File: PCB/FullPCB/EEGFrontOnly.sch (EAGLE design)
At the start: 208 parts, among them IC1 ADS1299-X, IC2 ADUM4160BRWZ, J11 MICRO-SD_CARD_SOCKET, J12 455-1750-1-ND, J13 455-1750-1-ND, J14 455-1750-1-ND, J15 455-1750-1-ND, J2 USB_B_PTH, J8 JTAG, U1 LP2985-33DBVT, U10 HT7318, U11 TMS320F28335PGFA, U12 HT7333, U13 2.93V, U14 MAX811-812, U2 B0505S-1WB0505S-1W, U3 TPS60403DBVT, U4 TPS73225DBVR, U5 TPS73225DBVR, U6 TPD4E1B06DCKR, U7 TPD4E1B06DCKR, U8 TPD4E1B06DCKR, U9 HT7333, Y1 30MHz, Y2 12MHz

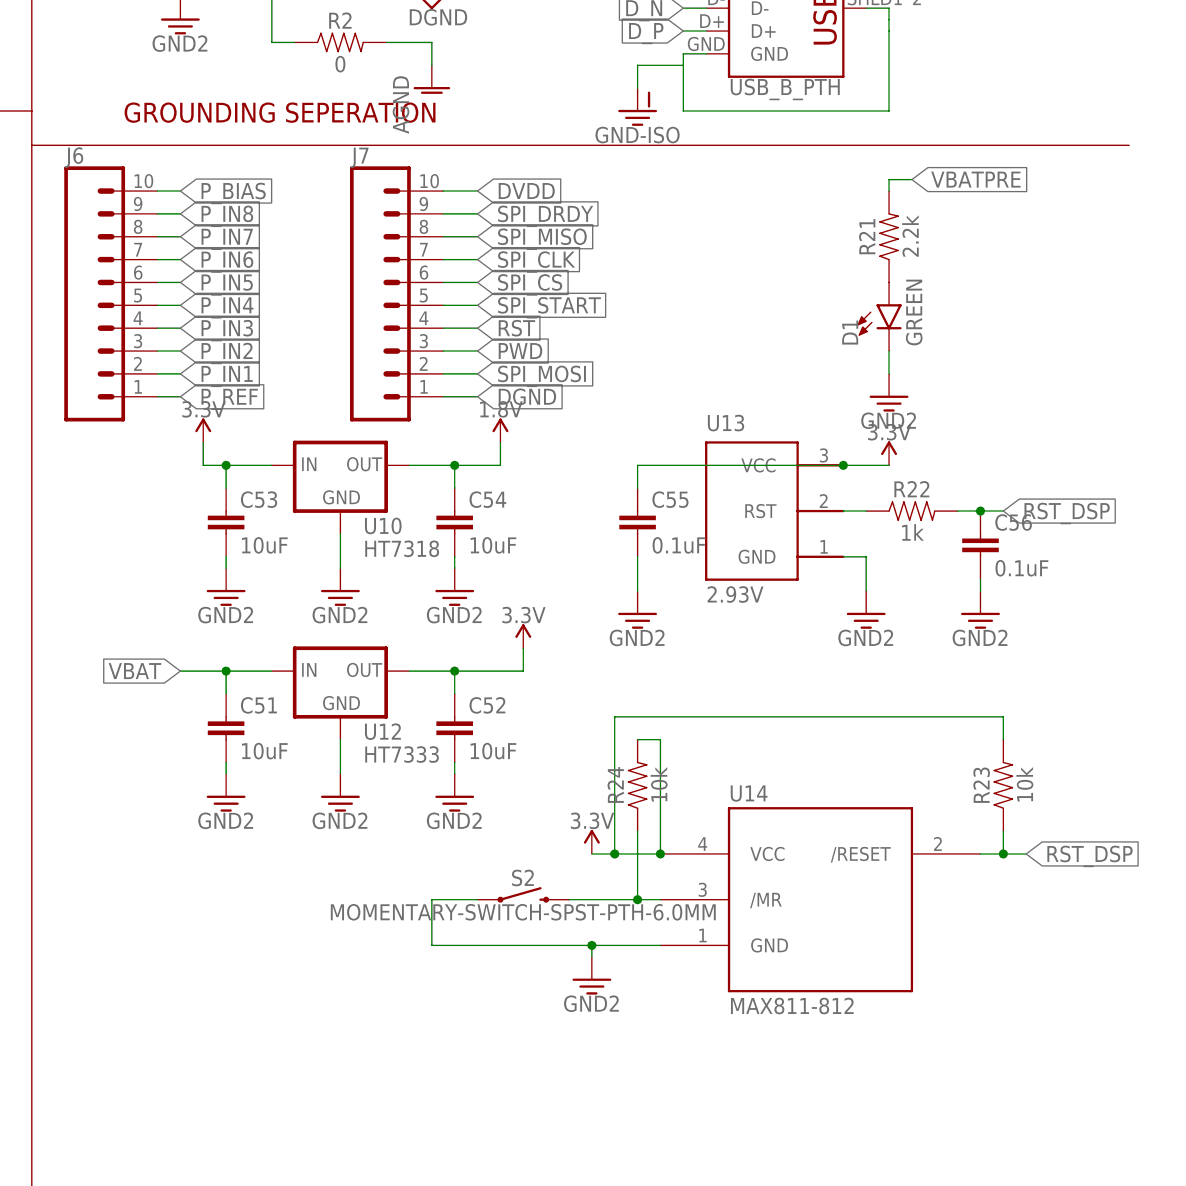
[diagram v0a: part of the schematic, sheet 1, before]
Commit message: full pcb nearly complete
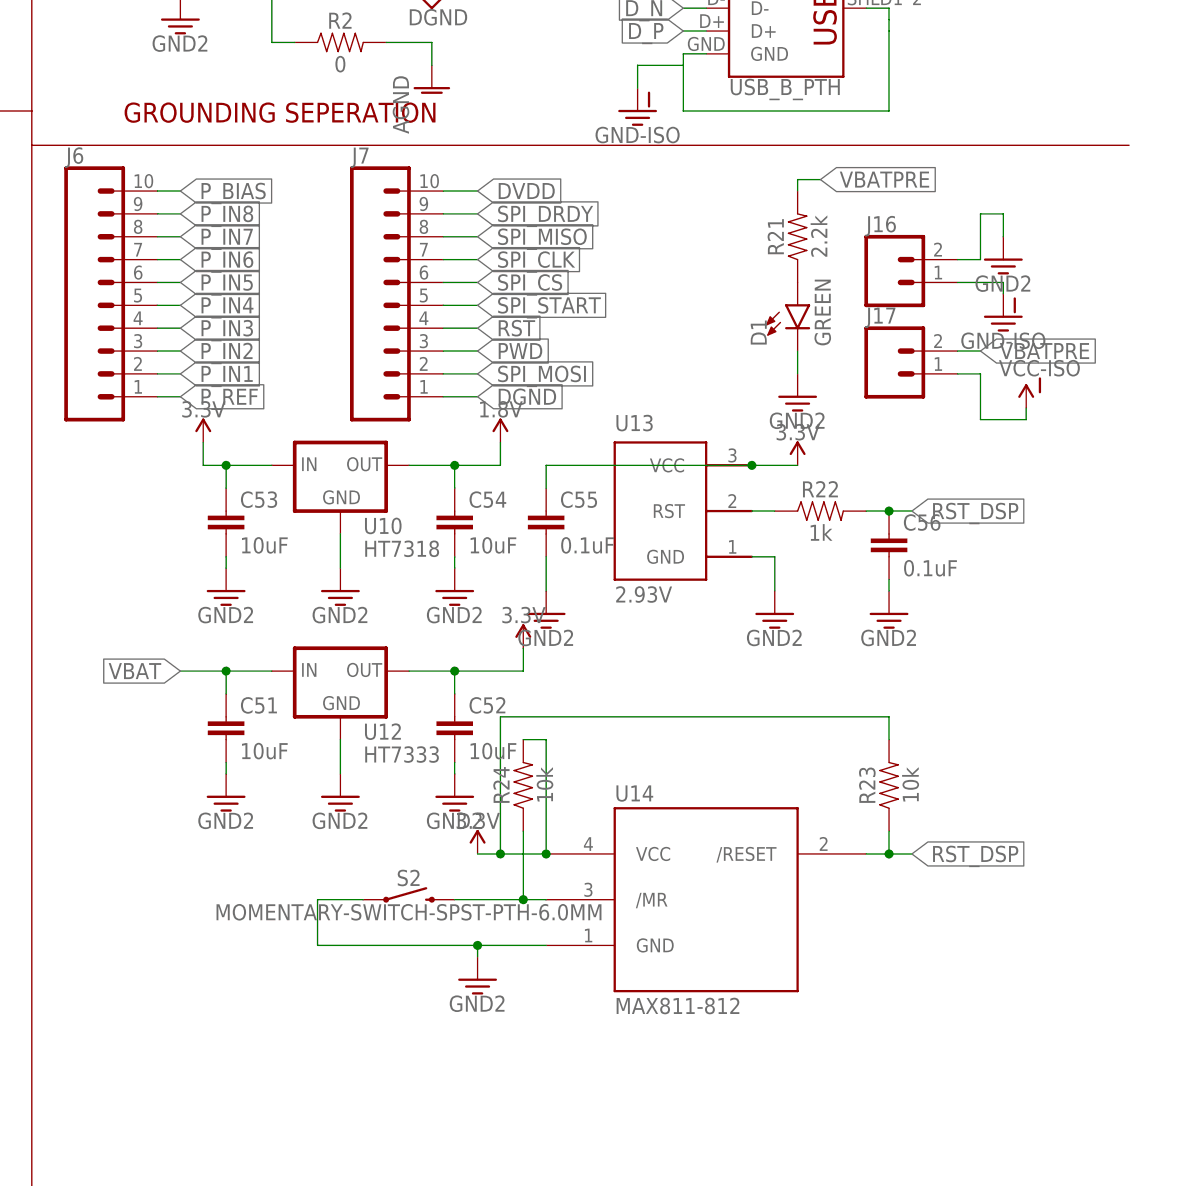
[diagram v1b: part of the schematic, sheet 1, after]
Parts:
- added J16, J17: (no value), SparkFun-Connectors:CONN_02
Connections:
- net GND: now also J16.2
- net GND-ISO: now also J16.1
- net VBATPRE: now also J17.2
- net VCC-ISO: now also J17.1
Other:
- moved on the sheet: C55, C56, D1, R21, R22, R23, R24, S2, U13, U14
